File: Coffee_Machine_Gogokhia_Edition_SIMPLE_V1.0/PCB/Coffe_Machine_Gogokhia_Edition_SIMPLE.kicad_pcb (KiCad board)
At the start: 2 copper layers, 108 x 49.5 mm, 98 parts, among them J1 LINE_TAB, J11 SW, J2 NEUT_TAB, J3 NTC, J4 BOILER_TAB, J5 PUMP_TAB, J6 SW1_TAB, J7 SW2_TAB, J8 FLOWMETER, J9 Conn_02x07_Counter_Clockwise, Q1 BTA16, Q2 BT131, Q3 BT131, Q4 BT131, U1 PC817, U2 PC817, U3 MOC3021M, U4 MOC3021M, U5 MOC3021M, U6 MOC3021M, U7 TLV1117-33, U8 LM4040DBZ-3, U9 STM32F103C8Tx, Y1 Crystal_GND24

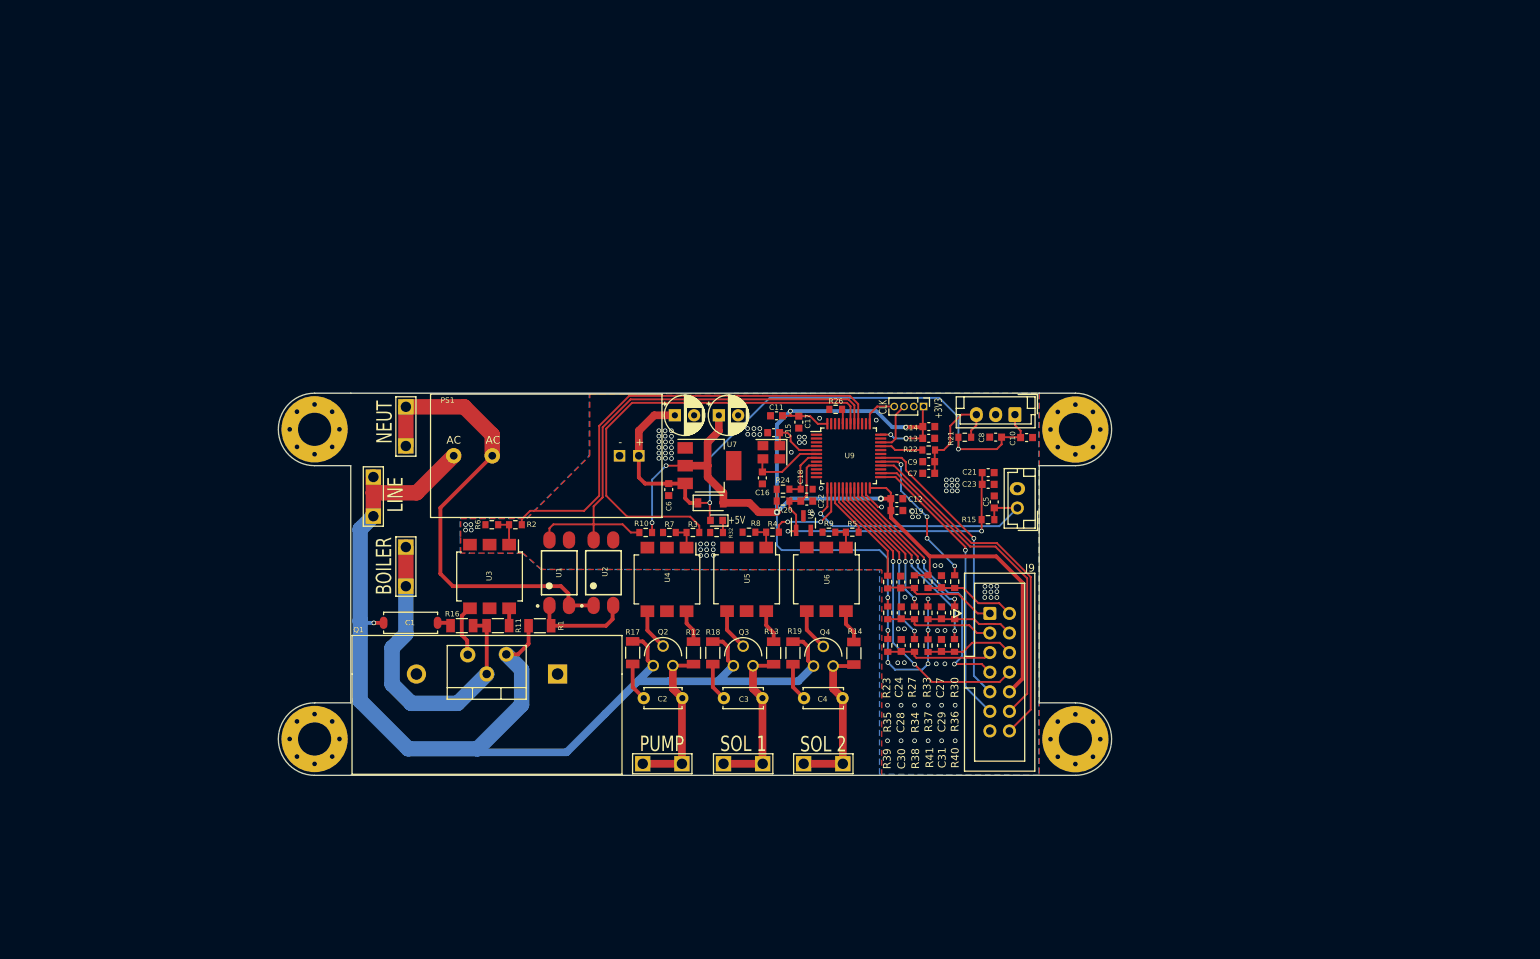
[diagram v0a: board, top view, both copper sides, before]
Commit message: Edited
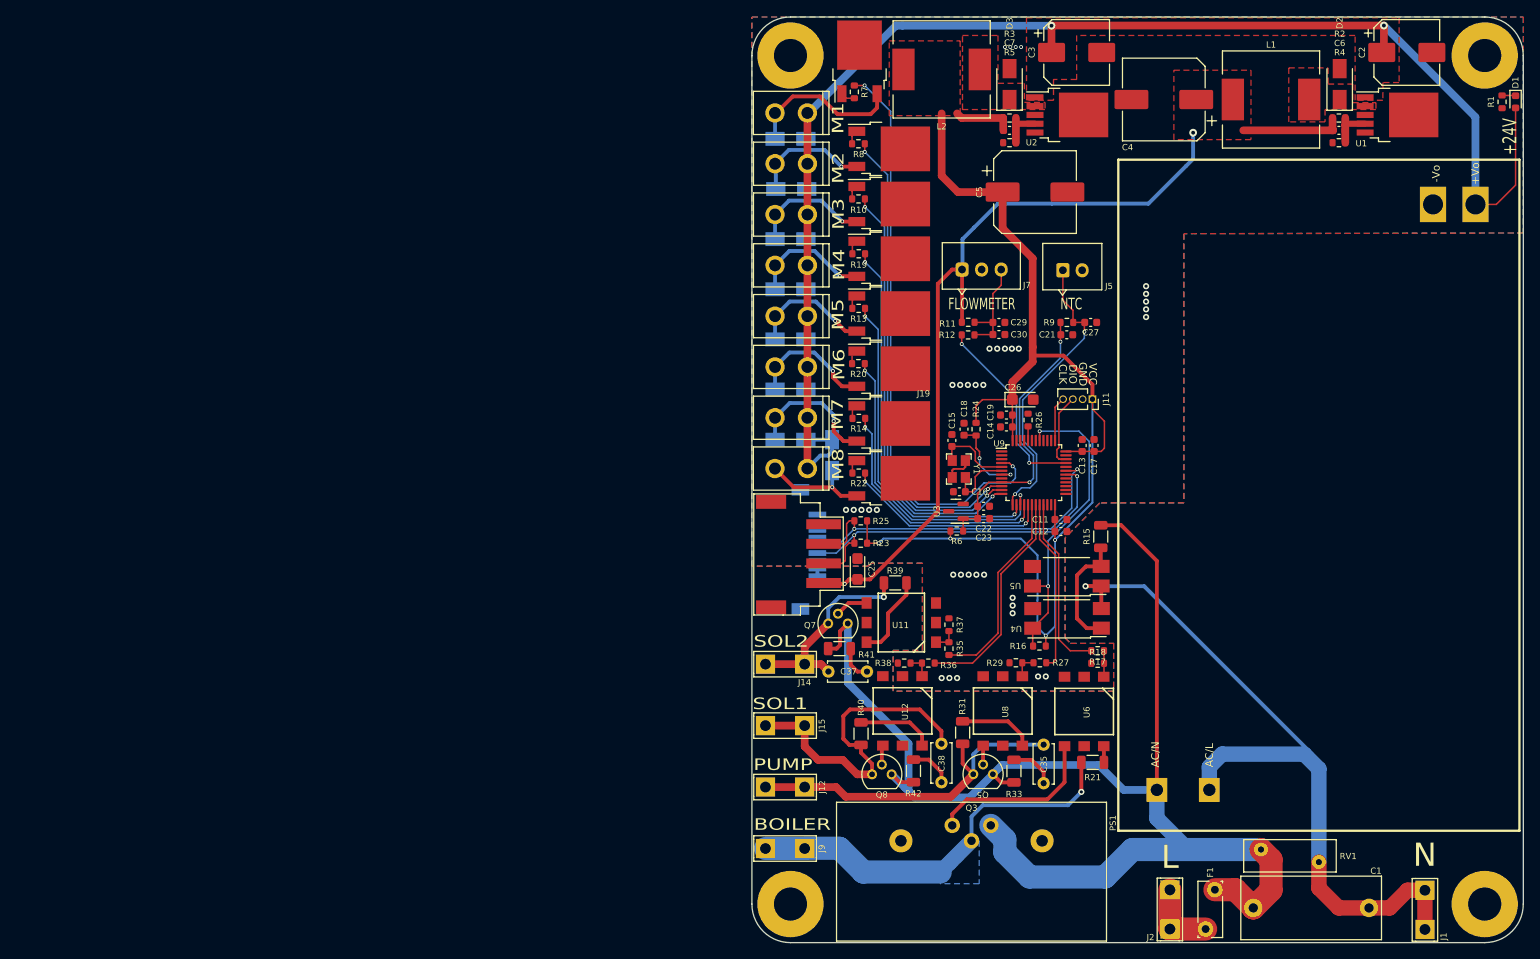
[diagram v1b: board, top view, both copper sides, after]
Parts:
- removed C10, C9: .01uF, MyLibrary:CAP_0603_^2
- removed C20: CP, Capacitor_THT:CP_Radial_D5.0mm_P2.50mm
- removed C24, C28, C31, C8: .1uF, MyLibrary:CAP_0603_^2
- removed R30, R32, R34: 1K, MyLibrary:RES_0603_^2
- removed the REF** at (93.3, 113.6)
- removed the REF** at (93.3, 73.5)
- removed the REF** at (191.9, 73.5)
- removed the REF** at (191.9, 113.6)
- removed U7: TLV1117-33, Package_TO_SOT_SMD:SOT-223-3_TabPin2
- added C26: 100uF, Capacitor_Tantalum_SMD:CP_EIA-3216-10_Kemet-I, F.Cu at (185.1, 69.6)
- added C35: .01uF, Capacitor_THT:C_Disc_D5.0mm_W2.5mm_P5.00mm, F.Cu at (187.8, 114.3)
- added C37: .01uF, Capacitor_THT:C_Disc_D5.0mm_W2.5mm_P5.00mm, F.Cu at (159.9, 104.9)
- added C38: .01uF, Capacitor_THT:C_Disc_D5.0mm_W2.5mm_P5.00mm, F.Cu at (174.6, 114.2)
- added D10: D, Diode_SMD:D_SMA, B.Cu at (155.0, 68.3)
- added D11: D, Diode_SMD:D_SMA, B.Cu at (160.4, 76.8)
- added D2: SS34, Diode_SMD:D_SMA, F.Cu at (226.2, 28.7)
- added D3: SS34, Diode_SMD:D_SMA, F.Cu at (183.4, 28.7)
- added D4: D, Diode_SMD:D_SMA, B.Cu at (155.0, 35.8)
- added D5: D, Diode_SMD:D_SMA, B.Cu at (155.1, 42.3)
- added D7: D, Diode_SMD:D_SMA, B.Cu at (155.0, 61.8)
- added D8: D, Diode_SMD:D_SMA, B.Cu at (155.0, 74.8)
- added D9: D, Diode_SMD:D_SMA, B.Cu at (155.0, 55.3)
- added F1: Fuse, Fuse:Fuse_Bourns_MF-RG300, F.Cu at (208.8, 138.2)
- added J10: Conn_01x02, Footprint:Molex_White_4_2mm_2P, F.Cu at (155.1, 72.1)
- added J12: PUMP_TAB, Footprint:TAB_Conn, F.Cu at (156.8, 119.8)
- added J13: Conn_01x02, Footprint:Molex_White_4_2mm_2P, F.Cu at (155.1, 52.3)
- added J14: SW1_TAB, Footprint:TAB_Conn, F.Cu at (156.8, 103.9)
- added J15: SW2_TAB, Footprint:TAB_Conn, F.Cu at (156.8, 111.9)
- added J16: Conn_01x02, Footprint:Molex_White_4_2mm_2P, F.Cu at (155.1, 65.5)
- added J17: Conn_01x02, Footprint:Molex_White_4_2mm_2P, F.Cu at (155.1, 78.6)
- added J18: Conn_01x10, Footprint:FCC_1.0mm_10P, B.Cu at (154.5, 89.0)
- added J19: SW, Footprint:XH2.54_4P_SMD, F.Cu at (156.0, 89.7)
- added L1: 47uH, Inductor_SMD:L_12x12mm_H8mm, F.Cu at (217.3, 30.7)
- added L2: 47uH, Inductor_SMD:L_12x12mm_H8mm, F.Cu at (174.6, 26.8)
- added Q10: 025N06N, Package_TO_SOT_SMD:TO-252-2, F.Cu at (167.8, 51.4)
- added Q11: 025N06N, Package_TO_SOT_SMD:TO-252-2, F.Cu at (167.8, 65.6)
- added Q12: 025N06N, Package_TO_SOT_SMD:TO-252-2, F.Cu at (167.8, 79.8)
- added Q5: BT131, Footprint:BT131, F.Cu at (180.0, 118.2)
- added Q6: 025N06N, Package_TO_SOT_SMD:TO-252-2, F.Cu at (167.8, 58.5)
- added Q7: BT131, Footprint:BT131, F.Cu at (161.2, 98.6)
- added Q8: BT131, Footprint:BT131, F.Cu at (166.8, 118.2)
- added Q9: 025N06N, Package_TO_SOT_SMD:TO-252-2, F.Cu at (167.8, 72.7)
- added R25: R, Resistor_SMD:R_0603_1608Metric, F.Cu at (164.1, 85.3)
- added R29: 10K, Resistor_SMD:R_0603_1608Metric, F.Cu at (184.2, 103.7)
- added R31: 180R, Resistor_SMD:R_1206_3216Metric, F.Cu at (177.3, 112.8)
- added R42: 39R, Resistor_SMD:R_1206_3216Metric, F.Cu at (170.9, 117.7)
- added REF**: MountingHole_4.3mm_M4_Pad, MountingHole:MountingHole_4.3mm_M4_Pad, F.Cu at (245.0, 135.0)
- added REF**: MountingHole_4.3mm_M4_Pad, MountingHole:MountingHole_4.3mm_M4_Pad, F.Cu at (155.0, 25.0)
- added REF**: MountingHole_4.3mm_M4_Pad, MountingHole:MountingHole_4.3mm_M4_Pad, F.Cu at (245.0, 25.0)
- added REF**: MountingHole_4.3mm_M4_Pad, MountingHole:MountingHole_4.3mm_M4_Pad, F.Cu at (155.0, 135.0)
- added RV1: Varistor, Varistor:RV_Disc_D12mm_W4.2mm_P7.5mm, F.Cu at (216.0, 127.9)
- added U11: MOC3021M, Footprint:DIP6_SMD, F.Cu at (169.4, 98.5)
- added U12: MOC3021M, Footprint:DIP6_SMD, F.Cu at (169.5, 110.0)
- C1: value .01uF -> 0.22uF; footprint Capacitor_THT:C_Disc_D5.0mm_W2.5mm_P5.00mm -> Capacitor_THT:C_Rect_L18.0mm_W8.0mm_P15.00mm_FKS3_FKP3
- C11, C12, C13, C14, C15, C16, C17, C18, C19, C21, C22, C23, C29: footprint MyLibrary:CAP_0603_^2 -> Capacitor_SMD:C_0603_1608Metric
- C2: value .01uF -> 100uF; footprint Capacitor_THT:C_Disc_D4.7mm_W2.5mm_P5.00mm -> Capacitor_SMD:CP_Elec_8x10
- C25: value CP -> 100uF; footprint Capacitor_THT:CP_Radial_D5.0mm_P2.50mm -> Capacitor_Tantalum_SMD:CP_EIA-3216-10_Kemet-I
- C27, C30: value .1uF -> .01uF; footprint MyLibrary:CAP_0603_^2 -> Capacitor_SMD:C_0603_1608Metric
- C3: value .01uF -> 100uF; footprint Capacitor_THT:C_Disc_D5.0mm_W2.5mm_P5.00mm -> Capacitor_SMD:CP_Elec_8x10
- C4: value .01uF -> 1000uF; footprint Capacitor_THT:C_Disc_D5.0mm_W2.5mm_P5.00mm -> Capacitor_SMD:CP_Elec_10x10.5
- C5: value .01uF -> 1000uF; footprint MyLibrary:CAP_0603_^2 -> Capacitor_SMD:CP_Elec_10x10.5
- C6, C7: value .1uF -> 15nF; footprint MyLibrary:CAP_0603_^2 -> Capacitor_SMD:C_0603_1608Metric
- D1: value D_Schottky -> LED; footprint Diode_SMD:D_SOD-123 -> LED_SMD:LED_0603_1608Metric
- D6: value LED -> D; footprint MyLibrary:LED_0603_^2 -> Diode_SMD:D_SMA; moved to B.Cu
- J1: value LINE_TAB -> NEUT_TAB; footprint MyLibrary:TAB_CONN -> Footprint:TAB_Conn
- J11: footprint Connector_PinHeader_1.27mm:PinHeader_1x04_P1.27mm_Vertical -> Connector_PinSocket_1.27mm:PinSocket_1x04_P1.27mm_Vertical
- J2: value NEUT_TAB -> LINE_TAB; footprint MyLibrary:TAB_CONN -> Footprint:TAB_Conn
- J3: value NTC -> Conn_01x02; footprint Connector_JST:JST_EH_B2B-EH-A_1x02_P2.50mm_Vertical -> Footprint:Molex_White_4_2mm_2P
- J4: value BOILER_TAB -> Conn_01x02; footprint MyLibrary:TAB_CONN -> Footprint:Molex_White_4_2mm_2P
- J5: value PUMP_TAB -> NTC; footprint MyLibrary:TAB_CONN -> Footprint:JST_2.54_2P
- J6: value SW1_TAB -> Conn_01x02; footprint MyLibrary:TAB_CONN -> Footprint:Molex_White_4_2mm_2P
- J7: value SW2_TAB -> FLOWMETER; footprint MyLibrary:TAB_CONN -> Footprint:JST_2.54_3P
- J8: value FLOWMETER -> Conn_01x02; footprint Connector_JST:JST_EH_B3B-EH-A_1x03_P2.50mm_Vertical -> Footprint:Molex_White_4_2mm_2P
- J9: value Conn_02x07_Counter_Clockwise -> BOILER_TAB; footprint Connector_IDC:IDC-Header_2x07_P2.54mm_Vertical -> Footprint:TAB_Conn
- PS1: footprint MyLibrary:HI_LINK_2W -> Footprint:IRM-90-24
- Q1: value BTA16 -> 025N06N; footprint Package_TO_SOT_THT:TO-220-3_Vertical -> Package_TO_SOT_SMD:TO-252-2
- Q2, Q4: value BT131 -> 025N06N; footprint MyLibrary:TO127P254X732-3 -> Package_TO_SOT_SMD:TO-252-2
- Q3: value BT131 -> BTA16; footprint MyLibrary:TO127P254X732-3 -> Footprint:BTA16_wH_SINK
- R1: value 100K -> 4.1K; footprint MyLibrary:RES_1206_^2 -> Resistor_SMD:R_0603_1608Metric
- R10, R7, R8: value 10K -> 1K; footprint MyLibrary:RES_0603_^2 -> Resistor_SMD:R_0603_1608Metric
- R11: value 180R -> 10K; footprint MyLibrary:RES_1206_^2 -> Resistor_SMD:R_0603_1608Metric
- R12, R13, R14: value 180R -> 1K; footprint MyLibrary:RES_1206_^2 -> Resistor_SMD:R_0603_1608Metric
- R15: value 47K -> 100K; footprint MyLibrary:RES_0603_^2 -> Resistor_SMD:R_1206_3216Metric
- R16, R18: value 39R -> 10K; footprint MyLibrary:RES_1206_^2 -> Resistor_SMD:R_0603_1608Metric
- R17: value 39R -> 330R; footprint MyLibrary:RES_1206_^2 -> Resistor_SMD:R_0603_1608Metric
- R19: value 39R -> 1K; footprint MyLibrary:RES_1206_^2 -> Resistor_SMD:R_0603_1608Metric
- R2: value 330R -> 3K; footprint MyLibrary:RES_0603_^2 -> Resistor_SMD:R_0603_1608Metric
- R20: value 33R -> 1K; footprint MyLibrary:RES_0603_^2 -> Resistor_SMD:R_0603_1608Metric
- R21, R39: value 10K -> 180R; footprint MyLibrary:RES_0603_^2 -> Resistor_SMD:R_1206_3216Metric
- R22, R24, R26, R37: footprint MyLibrary:RES_0603_^2 -> Resistor_SMD:R_0603_1608Metric
- R23: value 1K -> R; footprint MyLibrary:RES_0603_^2 -> Resistor_SMD:R_0603_1608Metric
- R27, R35: value 10K -> 330R; footprint MyLibrary:RES_0603_^2 -> Resistor_SMD:R_0603_1608Metric
- R3: value 330R -> 1.6K; footprint MyLibrary:RES_0603_^2 -> Resistor_SMD:R_0603_1608Metric
- R33, R41: value 10K -> 39R; footprint MyLibrary:RES_0603_^2 -> Resistor_SMD:R_1206_3216Metric
- R36: value 1K -> 330R; footprint MyLibrary:RES_0603_^2 -> Resistor_SMD:R_0603_1608Metric
- R38: value 1K -> 10K; footprint MyLibrary:RES_0603_^2 -> Resistor_SMD:R_0603_1608Metric
- R4, R5: value 330R -> 1K; footprint MyLibrary:RES_0603_^2 -> Resistor_SMD:R_0603_1608Metric
- R40: value 1K -> 180R; footprint MyLibrary:RES_0603_^2 -> Resistor_SMD:R_1206_3216Metric
- R6: value 10K -> 33R; footprint MyLibrary:RES_0603_^2 -> Resistor_SMD:R_0603_1608Metric
- R9: value 10K -> 47K; footprint MyLibrary:RES_0603_^2 -> Resistor_SMD:R_0603_1608Metric
- U1, U2: value PC817 -> LM2596T-ADJ; footprint MyLibrary:SOT254P975X400-4N -> Package_TO_SOT_SMD:TO-252-5_TabPin3
- U3: value MOC3021M -> LM4040DBZ-3; footprint MyLibrary:OPTOCOUPLER_H11F3SR2M -> Package_TO_SOT_SMD:SOT-23
- U4, U5: value MOC3021M -> PC817; footprint MyLibrary:OPTOCOUPLER_H11F3SR2M -> Footprint:PC817
- U6: footprint MyLibrary:OPTOCOUPLER_H11F3SR2M -> Footprint:DIP6_SMD
- U8: value LM4040DBZ-3 -> MOC3021M; footprint Package_TO_SOT_SMD:SOT-23 -> Footprint:DIP6_SMD
- Y1: footprint Crystal:Crystal_SMD_3225-4Pin_3.2x2.5mm -> Footprint:Crystal_smd_3225
- moved J1 147.4 mm to (237.2, 138.3)
- moved R1 142.0 mm to (247.2, 31.0), turned to 90 degrees
- moved C1 127.2 mm to (230.0, 135.5)
- moved C2 125.8 mm to (234.9, 24.6), turned to 0 degrees
- moved U1 123.8 mm to (233.7, 32.7), turned to 0 degrees
- moved R2 119.1 mm to (226.1, 33.1)
- moved D1 116.6 mm to (249.0, 31.0), turned to -90 degrees
- moved J2 115.9 mm to (204.2, 133.2)
- moved PS1 114.4 mm to (225.5, 83.5), turned to 90 degrees
- moved C6 98.6 mm to (226.1, 34.7), turned to 180 degrees
- moved C3 93.1 mm to (192.1, 24.6), turned to 0 degrees
- moved Q1 91.7 mm to (163.9, 25.8), turned to 90 degrees
- moved R4 89.1 mm to (226.1, 36.3), turned to 180 degrees
- moved C4 88.1 mm to (203.4, 30.7)
- moved U2 84.5 mm to (190.9, 32.7), turned to 0 degrees
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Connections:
- C1 pad 1: Net-(C1-Pad1) -> NEUT
- C2 pad 1: Net-(C2-Pad1) -> +24V
- C2 pad 2: Net-(C2-Pad2) -> GND
- C27 pad 1: DOWN_B -> NTC
- C29 pad 1: RIGHT_B -> Net-(C29-Pad1)
- C3 pad 1: Net-(C3-Pad1) -> +24V
- C3 pad 2: Net-(C3-Pad2) -> GND
- C30 pad 1: START_B -> Net-(C29-Pad1)
- C4 pad 1: Net-(C4-Pad1) -> +5V
- C4 pad 2: Net-(C4-Pad2) -> GND
- C5 pad 1: NTC -> +3V3
- C6 pad 1: +5V -> Net-(C6-Pad1)
- C6 pad 2: GND -> +5V
- C7 pad 2: GND -> +3V3
- D1 pad 1: +5V -> Net-(D1-Pad1)
- D1 pad 2: +3V3 -> +24V
- D6 pad 1: Net-(D6-Pad1) -> +24V
- D6 pad 2: +5V -> Net-(D6-Pad2)
- J1 pad 1: LINE -> NEUT
- J2 pad 1: NEUT -> Net-(F1-Pad1)
- J3 pad 1: NTC -> +24V
- J3 pad 2: GND -> Net-(D4-Pad2)
- J4 pad 1: Net-(J4-Pad1) -> +24V
- J5 pad 1: Net-(C2-Pad1) -> NTC
- J6 pad 1: Net-(C3-Pad1) -> +24V
- J7 pad 1: Net-(C4-Pad1) -> +5V
- J8 pad 1: +5V -> +24V
- J8 pad 2: GND -> Net-(D7-Pad2)
- J9 pad 1: UP_B -> Net-(J9-Pad1)
- PS1 pad 4: +5V -> +24V
- Q1 pad 1: LINE -> Net-(Q1-Pad1)
- Q1 pad 2: Net-(J4-Pad1) -> GND
- Q1 pad 3: Net-(Q1-Pad3) -> Net-(D4-Pad2)
- Q2 pad 1: LINE -> Net-(Q2-Pad1)
- Q2 pad 2: Net-(C2-Pad1) -> GND
- Q2 pad 3: Net-(Q2-Pad3) -> Net-(D5-Pad2)
- Q3 pad 2: Net-(C3-Pad1) -> Net-(J9-Pad1)
- Q4 pad 1: LINE -> Net-(Q4-Pad1)
- Q4 pad 2: Net-(C4-Pad1) -> GND
- Q4 pad 3: Net-(Q4-Pad3) -> Net-(D6-Pad2)
- R1 pad 1: Net-(R1-Pad1) -> GND
- R1 pad 2: LINE -> Net-(D1-Pad1)
- R10 pad 1: Z_CROSS -> Motor_3
- R10 pad 2: +3V3 -> Net-(Q4-Pad1)
- R11 pad 1: Net-(J4-Pad1) -> +5V
- R11 pad 2: Net-(R11-Pad2) -> Net-(C29-Pad1)
- R12 pad 1: Net-(C2-Pad1) -> Net-(C29-Pad1)
- R12 pad 2: Net-(R12-Pad2) -> FLOWMETER
- R13 pad 1: Net-(C3-Pad1) -> Motor_5
- R13 pad 2: Net-(R13-Pad2) -> Net-(Q6-Pad1)
- R14 pad 1: Net-(C4-Pad1) -> Motor_7
- R14 pad 2: Net-(R14-Pad2) -> Net-(Q9-Pad1)
- R15 pad 1: +3V0 -> Net-(R15-Pad1)
- R15 pad 2: NTC -> LINE
- R16 pad 1: Net-(C1-Pad1) -> Z_CROSS
- R16 pad 2: Net-(J4-Pad1) -> +3V3
- R17 pad 1: LINE -> Net-(R17-Pad1)
- R17 pad 2: Net-(C2-Pad2) -> BOILER_uC
- R18 pad 1: LINE -> GND
- R18 pad 2: Net-(C3-Pad2) -> Net-(R17-Pad1)
- R19 pad 1: LINE -> Motor_4
- R19 pad 2: Net-(C4-Pad2) -> Net-(Q10-Pad1)
- R2 pad 1: Net-(R2-Pad1) -> +5V
- R2 pad 2: BOILER_uC -> Net-(C6-Pad1)
- R20 pad 1: +3V0 -> Motor_6
- R20 pad 2: +3V3 -> Net-(Q11-Pad1)
- R21 pad 1: +5V -> Net-(J9-Pad1)
- R21 pad 2: Net-(C7-Pad1) -> Net-(R21-Pad2)
- R22 pad 1: Net-(C7-Pad1) -> Motor_8
- R22 pad 2: FLOWMETER -> Net-(Q12-Pad1)
- R23 pad 1: UP_B -> UART_Tx
- R23 pad 2: UP -> +3V3
- R27 pad 1: +3V3 -> Net-(R27-Pad1)
- R27 pad 2: UP_B -> PUMP_uC
- R3 pad 1: Net-(R3-Pad1) -> +3V3
- R3 pad 2: PUMP_uC -> Net-(C7-Pad1)
- R33 pad 1: +3V3 -> LINE
- R33 pad 2: DOWN_B -> Net-(C35-Pad2)
- R35 pad 1: +3V3 -> Net-(R35-Pad1)
- R35 pad 2: LEFT_B -> SW1_uC
- R36 pad 1: RIGHT_B -> Net-(R36-Pad1)
- R36 pad 2: RIGHT -> SW2_uC
- R37 pad 1: +3V3 -> GND
- R37 pad 2: RIGHT_B -> Net-(R35-Pad1)
- R38 pad 1: START_B -> GND
- R38 pad 2: START -> Net-(R36-Pad1)
- R39 pad 1: +3V3 -> Net-(C37-Pad1)
- R39 pad 2: START_B -> Net-(R39-Pad2)
- R4 pad 1: Net-(R4-Pad1) -> Net-(C6-Pad1)
- R4 pad 2: SW1_uC -> GND
- R40 pad 1: STOP_B -> Net-(C38-Pad1)
- R40 pad 2: STOP -> Net-(R40-Pad2)
- R41 pad 1: +3V3 -> LINE
- R41 pad 2: STOP_B -> Net-(C37-Pad2)
- R5 pad 1: Net-(R5-Pad1) -> Net-(C7-Pad1)
- R5 pad 2: SW2_uC -> GND
- R6 pad 1: GND -> +3V0
- R6 pad 2: Net-(R2-Pad1) -> +3V3
- R7 pad 1: GND -> Motor_1
- R7 pad 2: Net-(R3-Pad1) -> Net-(Q1-Pad1)
- R8 pad 1: GND -> Motor_2
- R8 pad 2: Net-(R4-Pad1) -> Net-(Q2-Pad1)
- R9 pad 1: GND -> +3V0
- R9 pad 2: Net-(R5-Pad1) -> NTC
- U1 pad 1: Net-(R1-Pad1) -> +24V
- U1 pad 2: NEUT -> Net-(D2-Pad1)
- U1 pad 4: Z_CROSS -> Net-(C6-Pad1)
- U2 pad 1: NEUT -> +24V
- U2 pad 2: Net-(R1-Pad1) -> Net-(D3-Pad1)
- U2 pad 4: Z_CROSS -> Net-(C7-Pad1)
- U3 pad 1: Net-(R2-Pad1) -> +3V0
- U3 pad 3: Net-(U3-Pad3) -> (no net)
- U4 pad 1: Net-(R3-Pad1) -> Net-(R15-Pad1)
- U4 pad 2: GND -> NEUT
- U4 pad 3: Net-(U4-Pad3) -> GND
- U4 pad 4: Net-(Q2-Pad3) -> Z_CROSS
- U5 pad 1: Net-(R4-Pad1) -> NEUT
- U5 pad 2: GND -> Net-(R15-Pad1)
- U5 pad 3: Net-(U5-Pad3) -> GND
- U5 pad 4: Net-(Q3-Pad3) -> Z_CROSS
- U6 pad 1: Net-(R5-Pad1) -> Net-(R17-Pad1)
- U6 pad 3: Net-(U6-Pad3) -> unconnected-(U6-Pad3)
- U6 pad 4: Net-(Q4-Pad3) -> Net-(Q3-Pad3)
- U6 pad 5: Net-(U6-Pad5) -> unconnected-(U6-Pad5)
- U6 pad 6: Net-(R14-Pad2) -> Net-(R21-Pad2)
- U8 pad 1: +3V0 -> Net-(R27-Pad1)
- U8 pad 3: (no net) -> unconnected-(U8-Pad3)
- U9 pad 1: Net-(U9-Pad1) -> unconnected-(U9-Pad1)
- U9 pad 10: Net-(U9-Pad10) -> Motor_2
- U9 pad 11: Net-(U9-Pad11) -> Motor_3
- U9 pad 12: Net-(U9-Pad12) -> Motor_4
- U9 pad 14: SW1_uC -> Motor_5
- U9 pad 15: SW2_uC -> Motor_6
- U9 pad 16: UP -> Motor_7
- U9 pad 17: RES -> Motor_8
- U9 pad 18: START -> SW1_uC
- U9 pad 19: LEFT -> SW2_uC
- U9 pad 2: Net-(U9-Pad2) -> unconnected-(U9-Pad2)
- U9 pad 20: STOP -> PUMP_uC
- U9 pad 21: RIGHT -> BOILER_uC
- U9 pad 22: DC -> unconnected-(U9-Pad22)
- U9 pad 25: SPI2_CS_SCREEN -> unconnected-(U9-Pad25)
- U9 pad 26: SPI2_SCK -> unconnected-(U9-Pad26)
- U9 pad 27: SPI2_MISO -> unconnected-(U9-Pad27)
- U9 pad 28: SPI2_MOSI -> unconnected-(U9-Pad28)
- U9 pad 29: DOWN -> unconnected-(U9-Pad29)
- U9 pad 3: Net-(U9-Pad3) -> unconnected-(U9-Pad3)
- U9 pad 30: SCREEN_LED -> UART_Tx
- U9 pad 31: Net-(U9-Pad31) -> UART_Rx
- U9 pad 32: Net-(U9-Pad32) -> unconnected-(U9-Pad32)
- U9 pad 38: Net-(U9-Pad38) -> unconnected-(U9-Pad38)
- U9 pad 39: Net-(U9-Pad39) -> unconnected-(U9-Pad39)
- U9 pad 4: Net-(U9-Pad4) -> Motor_1
- U9 pad 40: BOILER_uC -> unconnected-(U9-Pad40)
- U9 pad 42: PUMP_uC -> unconnected-(U9-Pad42)
- U9 pad 43: Net-(U9-Pad43) -> unconnected-(U9-Pad43)
- U9 pad 45: Net-(U9-Pad45) -> unconnected-(U9-Pad45)
- U9 pad 46: Net-(U9-Pad46) -> unconnected-(U9-Pad46)
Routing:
- net +24V: track 0.00 -> 208.9 mm, vias 0 -> 2
- net Motor_1: track 0.00 -> 75.8 mm, vias 0 -> 2
- net Motor_2: track 0.00 -> 62.0 mm, vias 0 -> 2
- net Motor_3: track 0.00 -> 55.3 mm, vias 0 -> 2
- net Net-(J9-Pad1): track 0.00 -> 52.2 mm, vias 0 -> 1
- net UART_Rx: track 0.00 -> 49.4 mm, vias 0 -> 2
- net UART_Tx: track 0.00 -> 48.9 mm, vias 0 -> 2
- net Motor_4: track 0.00 -> 48.7 mm, vias 0 -> 2
- net SPI2_MOSI: track 46.5 -> 0.00 mm
- net Net-(C35-Pad1): track 0.00 -> 45.4 mm
- net Motor_5: track 0.00 -> 44.2 mm, vias 0 -> 2
- net Net-(C38-Pad1): track 0.00 -> 43.9 mm
- net SPI2_SCK: track 42.8 -> 0.00 mm
- net Net-(J4-Pad1): track 41.4 -> 0.00 mm
- net Motor_6: track 0.00 -> 40.8 mm, vias 0 -> 2
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- added copper zone on F.Cu, net +24V
- added copper zone on F.Cu, net +3V3
- added copper zone on F.Cu, net +5V
- added copper zone on F.Cu, net Net-(D2-Pad1)
- added copper zone on F.Cu, net Net-(D3-Pad1)
- added copper zone on B.Cu, net Net-(J9-Pad1)
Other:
- board size 108 x 49.5 mm -> 100 x 120 mm
- board text added: "+24V"
- board text added: "DIO"
- board text added: "FLOWMETER"
- board text added: "GND"
- board text added: "L"
- board text added: "M1"
- board text added: "M2"
- board text added: "M3"
- board text added: "M4"
- board text added: "M5"
- board text added: "M6"
- board text added: "M7"
- board text added: "M8"
- board text added: "N"
- board text added: "NTC"
- board text added: "SOL1"
- board text added: "SOL2"
- board text added: "VCC"
- board text removed: "+3V3"
- board text removed: "+5V"
- board text removed: "LINE"
- board text removed: "MASTER GOGOKHIA EDITION"
- board text removed: "NEUT"
- board text removed: "SOL 1"
- board text removed: "SOL 2"

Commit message: 1
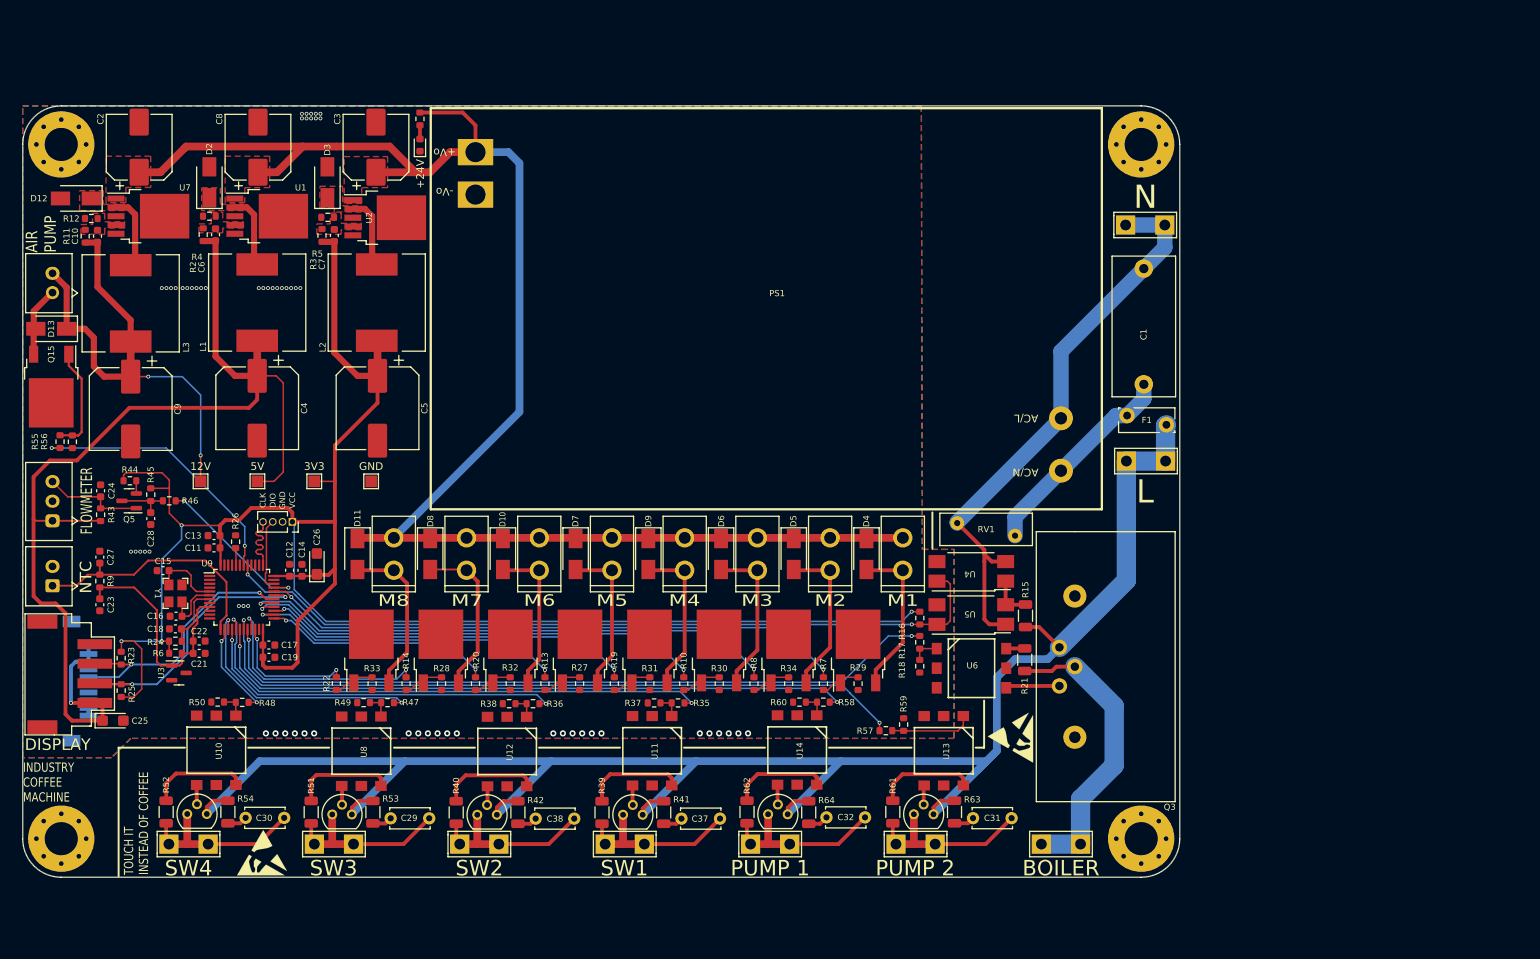
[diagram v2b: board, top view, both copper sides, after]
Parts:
- removed C35: .01uF, Capacitor_THT:C_Disc_D5.0mm_W2.5mm_P5.00mm
- removed the REF** at (245.0, 135.0)
- removed the REF** at (155.0, 25.0)
- removed the REF** at (245.0, 25.0)
- removed the REF** at (155.0, 135.0)
- added 12V: TestPoint_Pad_1.5x1.5mm, TestPoint:TestPoint_Pad_1.5x1.5mm, F.Cu at (78.5, 80.2)
- added 3V3: TestPoint_Pad_1.5x1.5mm, TestPoint:TestPoint_Pad_1.5x1.5mm, F.Cu at (93.3, 80.2)
- added 5V: TestPoint_Pad_1.5x1.5mm, TestPoint:TestPoint_Pad_1.5x1.5mm, F.Cu at (85.9, 80.2)
- added C10: 15nF, Capacitor_SMD:C_0603_1608Metric, F.Cu at (65.2, 48.4)
- added C24: 0.1uF, Capacitor_SMD:C_0603_1608Metric, F.Cu at (65.6, 81.4)
- added C28: 0.1uF, Capacitor_SMD:C_0603_1608Metric, F.Cu at (72.1, 85.0)
- added C31: .01uF, Capacitor_THT:C_Disc_D5.0mm_W2.5mm_P5.00mm, F.Cu at (183.7, 123.9)
- added C32: .01uF, Capacitor_THT:C_Disc_D5.0mm_W2.5mm_P5.00mm, F.Cu at (164.7, 123.8)
- added C8: 100uF, Capacitor_SMD:CP_Elec_8x10, F.Cu at (86.0, 36.9)
- added C9: 1000uF, Capacitor_SMD:CP_Elec_10x10.5, F.Cu at (69.5, 70.8)
- added D12: SS34, Diode_SMD:D_SMA, F.Cu at (62.4, 43.5)
- added D13: D, Diode_SMD:D_SMA, F.Cu at (59.2, 60.4)
- added GND: TestPoint_Pad_1.5x1.5mm, TestPoint:TestPoint_Pad_1.5x1.5mm, F.Cu at (100.6, 80.2)
- added J20: SW4_TAB, Footprint:TAB_Conn, F.Cu at (74.4, 127.2)
- added J21: Conn_01x02, Footprint:JST_2.54_2P, F.Cu at (59.2, 54.7)
- added J22: PUMP1_TAB, Footprint:TAB_Conn, F.Cu at (168.7, 127.2)
- added J23: PUMP2_TAB, Footprint:TAB_Conn, F.Cu at (149.8, 127.2)
- added L3: 47uH, Inductor_SMD:L_12x12mm_H8mm, F.Cu at (69.5, 57.1)
- added Q13: BT131, Footprint:BT131, F.Cu at (96.9, 123.4)
- added Q14: BT131, Footprint:BT131, F.Cu at (78.1, 123.3)
- added Q15: 025N06N, Package_TO_SOT_SMD:TO-252-2, F.Cu at (59.2, 67.9)
- added Q16: BT131, Footprint:BT131, F.Cu at (172.3, 123.4)
- added Q17: BT131, Footprint:BT131, F.Cu at (153.4, 123.4)
- added R28: 10K, Resistor_SMD:R_0603_1608Metric, F.Cu at (109.8, 106.4)
- added R30: 10K, Resistor_SMD:R_0603_1608Metric, F.Cu at (145.8, 106.4)
- added R32: 10K, Resistor_SMD:R_0603_1608Metric, F.Cu at (118.7, 106.4)
- added R34: 10K, Resistor_SMD:R_0603_1608Metric, F.Cu at (154.8, 106.4)
- added R43: 10k, Resistor_SMD:R_0603_1608Metric, F.Cu at (65.6, 84.5)
- added R44: 1k, Resistor_SMD:R_0603_1608Metric, F.Cu at (69.4, 80.1)
- added R45: 10k, Resistor_SMD:R_0603_1608Metric, F.Cu at (72.1, 81.9)
- added R46: 1k, Resistor_SMD:R_0603_1608Metric, F.Cu at (74.5, 82.7)
- added R47: 330R, Resistor_SMD:R_0603_1608Metric, F.Cu at (102.8, 108.9)
- added R48: 330R, Resistor_SMD:R_0603_1608Metric, F.Cu at (83.9, 108.9)
- added R49: 10K, Resistor_SMD:R_0603_1608Metric, F.Cu at (99.7, 108.9)
- added R50: 10K, Resistor_SMD:R_0603_1608Metric, F.Cu at (80.7, 108.8)
- added R51: 180R, Resistor_SMD:R_1206_3216Metric, F.Cu at (92.9, 123.1)
- added R52: 180R, Resistor_SMD:R_1206_3216Metric, F.Cu at (74.1, 123.1)
- added R53: 39R, Resistor_SMD:R_1206_3216Metric, F.Cu at (100.9, 123.1)
- added R54: 39R, Resistor_SMD:R_1206_3216Metric, F.Cu at (82.1, 123.1)
- added R55: 1K, Resistor_SMD:R_0603_1608Metric, F.Cu at (60.3, 75.0)
- added R56: 10K, Resistor_SMD:R_0603_1608Metric, F.Cu at (61.9, 75.1)
- added R57: 330R, Resistor_SMD:R_0603_1608Metric, F.Cu at (167.4, 112.5)
- added R58: 330R, Resistor_SMD:R_0603_1608Metric, F.Cu at (159.3, 108.8)
- added R59: 10K, Resistor_SMD:R_0603_1608Metric, F.Cu at (169.7, 111.7)
- added R60: 10K, Resistor_SMD:R_0603_1608Metric, F.Cu at (156.2, 108.8)
- added R61: 180R, Resistor_SMD:R_1206_3216Metric, F.Cu at (168.3, 123.1)
- added R62: 180R, Resistor_SMD:R_1206_3216Metric, F.Cu at (149.4, 123.1)
- added R63: 39R, Resistor_SMD:R_1206_3216Metric, F.Cu at (176.3, 123.1)
- added R64: 39R, Resistor_SMD:R_1206_3216Metric, F.Cu at (157.4, 123.1)
- added REF**: MountingHole_4.3mm_M4_Pad_Via, MountingHole:MountingHole_4.3mm_M4_Pad_Via, F.Cu at (60.5, 36.5)
- added REF**: ESD-Logo_6.6x6mm_SilkScreen, Symbol:ESD-Logo_6.6x6mm_SilkScreen, F.Cu at (86.5, 128.3)
- added REF**: ESD-Logo_6.6x6mm_SilkScreen, Symbol:ESD-Logo_6.6x6mm_SilkScreen, F.Cu at (183.5, 113.4)
- added REF**: MountingHole_4.3mm_M4_Pad_Via, MountingHole:MountingHole_4.3mm_M4_Pad_Via, F.Cu at (60.5, 126.5)
- added REF**: MountingHole_4.3mm_M4_Pad_Via, MountingHole:MountingHole_4.3mm_M4_Pad_Via, F.Cu at (200.5, 126.5)
- added REF**: MountingHole_4.3mm_M4_Pad_Via, MountingHole:MountingHole_4.3mm_M4_Pad_Via, F.Cu at (200.5, 36.5)
- added U10: MOC3021M, Footprint:DIP6_SMD, F.Cu at (80.6, 115.1)
- added U13: MOC3021M, Footprint:DIP6_SMD, F.Cu at (174.9, 115.1)
- added U14: MOC3021M, Footprint:DIP6_SMD, F.Cu at (155.9, 115.0)
- added U7: LM2596T-ADJ, Package_TO_SOT_SMD:TO-252-5_TabPin3, F.Cu at (71.8, 45.8)
- C29: value .1uF -> .01uF; footprint Capacitor_SMD:C_0603_1608Metric -> Capacitor_THT:C_Disc_D5.0mm_W2.5mm_P5.00mm
- C30: footprint Capacitor_SMD:C_0603_1608Metric -> Capacitor_THT:C_Disc_D5.0mm_W2.5mm_P5.00mm
- D10, D11, D4, D5, D6, D7, D8, D9: moved to F.Cu
- J12: value PUMP_TAB -> SW3_TAB
- J7: value FLOWMETER -> JST_3P_2.54mm
- Q5: value BT131 -> 2N2222; footprint Footprint:BT131 -> Package_TO_SOT_SMD:SOT-23
- R11: value 10K -> 11K
- R12: value 1K -> 1.2K
- R27: value 330R -> 10K
- R31: value 180R -> 10K; footprint Resistor_SMD:R_1206_3216Metric -> Resistor_SMD:R_0603_1608Metric
- R33: value 39R -> 10K; footprint Resistor_SMD:R_1206_3216Metric -> Resistor_SMD:R_0603_1608Metric
- R9: value 47K -> 100K
- moved C2 164.8 mm to (70.6, 36.9), turned to 90 degrees
- moved R2 148.0 mm to (78.9, 48.2), turned to 90 degrees
- moved U1 147.1 mm to (87.2, 45.8)
- moved D2 147.1 mm to (79.7, 41.4)
- moved R4 146.7 mm to (79.7, 45.8)
- moved C6 146.3 mm to (80.5, 48.2), turned to -90 degrees
- moved D1 142.1 mm to (107.0, 36.6), turned to 90 degrees
- moved R1 140.3 mm to (107.0, 33.2)
- moved J5 138.0 mm to (59.2, 92.7), turned to 90 degrees
- moved L1 134.0 mm to (85.9, 57.0), turned to -90 degrees
- moved C27 132.0 mm to (65.5, 90.0), turned to 90 degrees
- moved R9 129.8 mm to (65.5, 93.1), turned to 90 degrees
- moved C4 124.2 mm to (85.9, 70.7), turned to -90 degrees
- moved J7 122.3 mm to (59.3, 85.3), turned to 90 degrees
- moved C21 119.8 mm to (78.3, 102.5)
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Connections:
- net OSC_IN renamed Net-(C15-Pad2)
- net OSC_OUT renamed Net-(C16-Pad2)
- C1 pad 2: LINE -> Net-(C1-Pad2)
- C29 pad 2: GND -> Net-(C29-Pad2)
- C30 pad 1: Net-(C29-Pad1) -> Net-(C30-Pad1)
- C30 pad 2: GND -> Net-(C30-Pad2)
- D1 pad 1: Net-(D1-Pad1) -> GND
- D1 pad 2: +24V -> Net-(D1-Pad2)
- F1 pad 1: Net-(F1-Pad1) -> LINE
- F1 pad 2: LINE -> Net-(C1-Pad2)
- J10 pad 1: +24V -> Net-(D8-Pad2)
- J10 pad 2: Net-(D8-Pad2) -> +24V
- J12 pad 1: Net-(C35-Pad1) -> Net-(C29-Pad1)
- J13 pad 1: +24V -> Net-(D9-Pad2)
- J13 pad 2: Net-(D9-Pad2) -> +24V
- J16 pad 1: +24V -> Net-(D10-Pad2)
- J16 pad 2: Net-(D10-Pad2) -> +24V
- J17 pad 1: +24V -> Net-(D11-Pad2)
- J17 pad 2: Net-(D11-Pad2) -> +24V
- J18 pad 1: GND -> +5V
- J18 pad 10: +5V -> GND
- J18 pad 2: GND -> +5V
- J18 pad 3: GND -> +5V
- J18 pad 5: UART_Rx -> UART_Tx
- J18 pad 6: UART_Tx -> UART_Rx
- J18 pad 8: +5V -> GND
- J18 pad 9: +5V -> GND
- J19 pad 2: UART_Tx -> UART_Rx
- J19 pad 3: UART_Rx -> UART_Tx
- J2 pad 1: Net-(F1-Pad1) -> LINE
- J3 pad 1: +24V -> Net-(D4-Pad2)
- J3 pad 2: Net-(D4-Pad2) -> +24V
- J4 pad 1: +24V -> Net-(D5-Pad2)
- J4 pad 2: Net-(D5-Pad2) -> +24V
- J6 pad 1: +24V -> Net-(D6-Pad2)
- J6 pad 2: Net-(D6-Pad2) -> +24V
- J7 pad 3: Net-(C29-Pad1) -> Net-(C24-Pad2)
- J8 pad 1: +24V -> Net-(D7-Pad2)
- J8 pad 2: Net-(D7-Pad2) -> +24V
- PS1 pad 1: LINE -> Net-(C1-Pad2)
- Q5 pad 1: LINE -> Net-(C24-Pad2)
- Q5 pad 2: Net-(C35-Pad1) -> Net-(Q5-Pad2)
- Q5 pad 3: Net-(Q5-Pad3) -> Net-(C28-Pad2)
- R1 pad 1: GND -> Net-(D1-Pad2)
- R1 pad 2: Net-(D1-Pad1) -> +24V
- R11 pad 1: +5V -> +12V
- R11 pad 2: Net-(C29-Pad1) -> Net-(C10-Pad1)
- R12 pad 1: Net-(C29-Pad1) -> Net-(C10-Pad1)
- R12 pad 2: FLOWMETER -> GND
- R27 pad 1: Net-(R27-Pad1) -> Net-(Q6-Pad1)
- R27 pad 2: PUMP_uC -> GND
- R29 pad 1: GND -> Net-(Q1-Pad1)
- R29 pad 2: Net-(R27-Pad1) -> GND
- R31 pad 1: Net-(C35-Pad1) -> Net-(Q10-Pad1)
- R31 pad 2: Net-(R31-Pad2) -> GND
- R33 pad 1: LINE -> Net-(Q12-Pad1)
- R33 pad 2: Net-(C35-Pad2) -> GND
- RV1 pad 1: LINE -> Net-(C1-Pad2)
- U8 pad 1: Net-(R27-Pad1) -> Net-(R47-Pad1)
- U8 pad 4: Net-(Q5-Pad3) -> Net-(Q13-Pad3)
- U8 pad 6: Net-(R31-Pad2) -> Net-(R51-Pad2)
- U9 pad 10: Motor_2 -> unconnected-(U9-Pad10)
- U9 pad 11: Motor_3 -> unconnected-(U9-Pad11)
- U9 pad 12: Motor_4 -> unconnected-(U9-Pad12)
- U9 pad 14: Motor_5 -> SW4_uC
- U9 pad 15: Motor_6 -> SW3_uC
- U9 pad 16: Motor_7 -> SW2_uC
- U9 pad 17: Motor_8 -> SW1_uC
- U9 pad 18: SW1_uC -> PUMP2_uC
- U9 pad 19: SW2_uC -> PUMP1_uC
- U9 pad 20: PUMP_uC -> BOILER_uC
- U9 pad 21: BOILER_uC -> Motor_7
- U9 pad 22: unconnected-(U9-Pad22) -> Motor_8
- U9 pad 25: unconnected-(U9-Pad25) -> Motor_6
- U9 pad 26: unconnected-(U9-Pad26) -> Motor_5
- U9 pad 27: unconnected-(U9-Pad27) -> Motor_4
- U9 pad 28: unconnected-(U9-Pad28) -> Motor_3
- U9 pad 29: unconnected-(U9-Pad29) -> Motor_2
- U9 pad 32: unconnected-(U9-Pad32) -> Motor_1
- U9 pad 4: Motor_1 -> unconnected-(U9-Pad4)
- U9 pad 42: unconnected-(U9-Pad42) -> AIR_PUMP_uC
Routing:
- net PUMP1_uC: track 0.00 -> 93.8 mm, vias 0 -> 2
- net +3V3: track 168.3 -> 261.8 mm
- net PUMP2_uC: track 0.00 -> 85.3 mm, vias 0 -> 2
- net BOILER_uC: track 23.1 -> 95.3 mm, vias 0 -> 2
- net +12V: track 0.00 -> 63.1 mm, vias 0 -> 2
- net Z_CROSS: track 39.8 -> 101.8 mm
- net LINE: track 182.7 -> 244.2 mm
- net Net-(C35-Pad1): track 45.4 -> 0.00 mm
- net SW1_uC: track 26.0 -> 69.9 mm, vias 0 -> 2
- net AIR_PUMP_uC: track 0.00 -> 35.4 mm, vias 0 -> 2
- net SW3_uC: track 0.00 -> 33.1 mm, vias 0 -> 2
- net Net-(C1-Pad2): track 0.00 -> 27.4 mm
- net +5V: track 119.4 -> 146.2 mm, vias 2 -> 1
- net NEUT: track 98.3 -> 75.0 mm, vias 1 -> 0
- net Net-(C31-Pad1): track 0.00 -> 23.2 mm
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- added copper zone on F.Cu, net Net-(C10-Pad1)
- added copper zone on F.Cu, net Net-(C6-Pad1)
- added copper zone on F.Cu, net Net-(C7-Pad1)
- added copper zone on F.Cu, net Net-(D12-Pad1)
- removed copper zone on F.Cu, net +3V3
- removed copper zone on F.Cu, net +5V
- removed copper zone on B.Cu, net Net-(J9-Pad1)
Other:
- board size 100 x 120 mm -> 150 x 100 mm
- board text added: "AIR PUMP"
- board text added: "DISPLAY"
- board text added: "INDUSTRY COFFEE MACHINE"
- board text added: "PUMP 1"
- board text added: "PUMP 2"
- board text added: "SW1"
- board text added: "SW2"
- board text added: "SW3"
- board text added: "SW4"
- board text added: "TOUCH IT INSTEAD OF COFFEE"
- board text removed: "PUMP"
- board text removed: "SOL1"
- board text removed: "SOL2"
